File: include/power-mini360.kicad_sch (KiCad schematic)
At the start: 4 parts, among them U4 MINI360

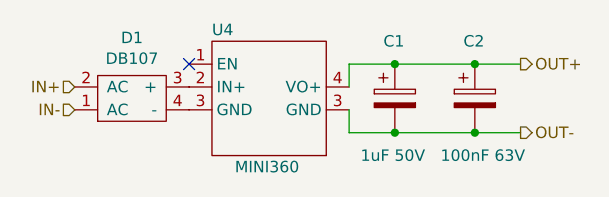
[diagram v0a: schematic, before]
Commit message: refactor master-wt32
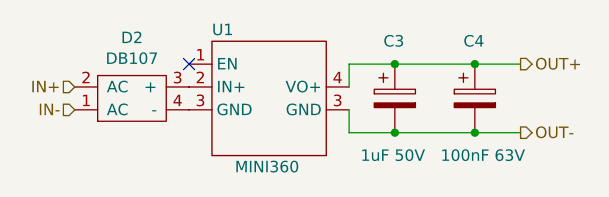
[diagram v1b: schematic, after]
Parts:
- renumbered C1 to C3, C2 to C4, D1 to D2, U4 to U1
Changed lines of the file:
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@@
   (symbol (lib_id "Device:C_Polarized") (at 66.04 30.48 0)
     (in_bom yes) (on_board yes)
-    (property "Reference" "C1" (id 0) (at 64.77 24.13 0)
+    (property "Reference" "C3" (id 0) (at 64.77 24.13 0)
       (effects (font (size 1.27 1.27)) (justify left))
     )
@@
   (symbol (lib_id "Device:C_Polarized") (at 74.93 30.48 0)
     (in_bom yes) (on_board yes)
-    (property "Reference" "C2" (id 0) (at 73.66 24.13 0)
+    (property "Reference" "C4" (id 0) (at 73.66 24.13 0)
       (effects (font (size 1.27 1.27)) (justify left))
     )
@@
   (symbol (lib_id "custom:DB107") (at 36.83 30.48 0) (mirror x)
     (in_bom yes) (on_board yes)
-    (property "Reference" "D1" (id 0) (at 36.83 23.749 0))
+    (property "Reference" "D2" (id 0) (at 36.83 23.749 0))
     (property "Value" "DB107" (id 1) (at 36.83 26.0604 0))
     (property "Footprint" "custom:DB107" (id 2) (at 36.83 24.13 0)
@@
   (symbol (lib_id "boards:MINI360") (at 52.07 30.48 0)
     (in_bom yes) (on_board yes)
-    (property "Reference" "U4" (id 0) (at 45.72 22.8599 0)
+    (property "Reference" "U1" (id 0) (at 45.72 22.8599 0)
       (effects (font (size 1.27 1.27)) (justify left))
     )

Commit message: refactor master-wt32 pcb
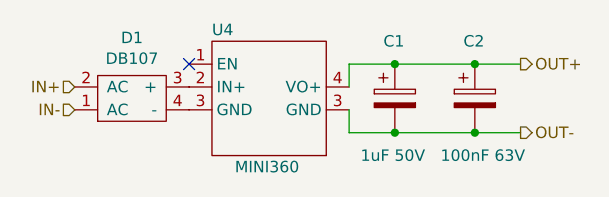
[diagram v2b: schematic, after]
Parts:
- renumbered C3 to C1, C4 to C2, D2 to D1, U1 to U4
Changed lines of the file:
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@@
   (symbol (lib_id "Device:C_Polarized") (at 66.04 30.48 0)
     (in_bom yes) (on_board yes)
-    (property "Reference" "C3" (id 0) (at 64.77 24.13 0)
+    (property "Reference" "C1" (id 0) (at 64.77 24.13 0)
       (effects (font (size 1.27 1.27)) (justify left))
     )
@@
   (symbol (lib_id "Device:C_Polarized") (at 74.93 30.48 0)
     (in_bom yes) (on_board yes)
-    (property "Reference" "C4" (id 0) (at 73.66 24.13 0)
+    (property "Reference" "C2" (id 0) (at 73.66 24.13 0)
       (effects (font (size 1.27 1.27)) (justify left))
     )
@@
   (symbol (lib_id "custom:DB107") (at 36.83 30.48 0) (mirror x)
     (in_bom yes) (on_board yes)
-    (property "Reference" "D2" (id 0) (at 36.83 23.749 0))
+    (property "Reference" "D1" (id 0) (at 36.83 23.749 0))
     (property "Value" "DB107" (id 1) (at 36.83 26.0604 0))
     (property "Footprint" "custom:DB107" (id 2) (at 36.83 24.13 0)
@@
   (symbol (lib_id "boards:MINI360") (at 52.07 30.48 0)
     (in_bom yes) (on_board yes)
-    (property "Reference" "U1" (id 0) (at 45.72 22.8599 0)
+    (property "Reference" "U4" (id 0) (at 45.72 22.8599 0)
       (effects (font (size 1.27 1.27)) (justify left))
     )
